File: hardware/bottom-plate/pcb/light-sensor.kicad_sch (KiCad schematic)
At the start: 4 parts

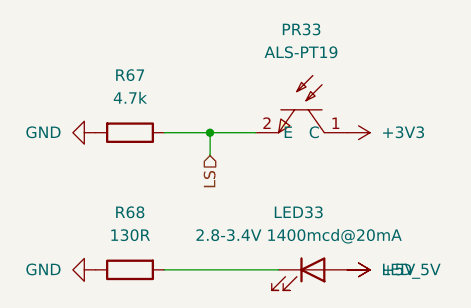
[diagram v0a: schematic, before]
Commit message: actually fixed it (merging moment)
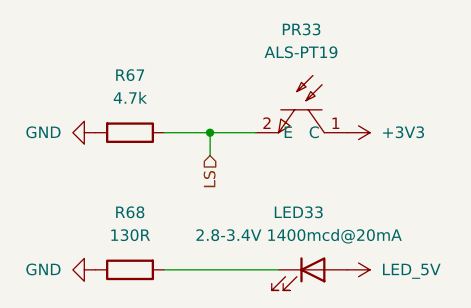
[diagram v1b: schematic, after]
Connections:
- net +5V renamed LED_5V
